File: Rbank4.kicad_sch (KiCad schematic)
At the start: 100 parts, among them K10 TQ2-5, K11 TQ2-5, K12 TQ2-5, K13 TQ2-5, K14 TQ2-5, K15 TQ2-5, K16 TQ2-5, K17 TQ2-5, K18 TQ2-5, Q10 2N2222, Q11 2N2222, Q12 2N2222, Q13 2N2222, Q14 2N2222, Q15 2N2222, Q16 2N2222, Q17 2N2222, Q18 2N2222

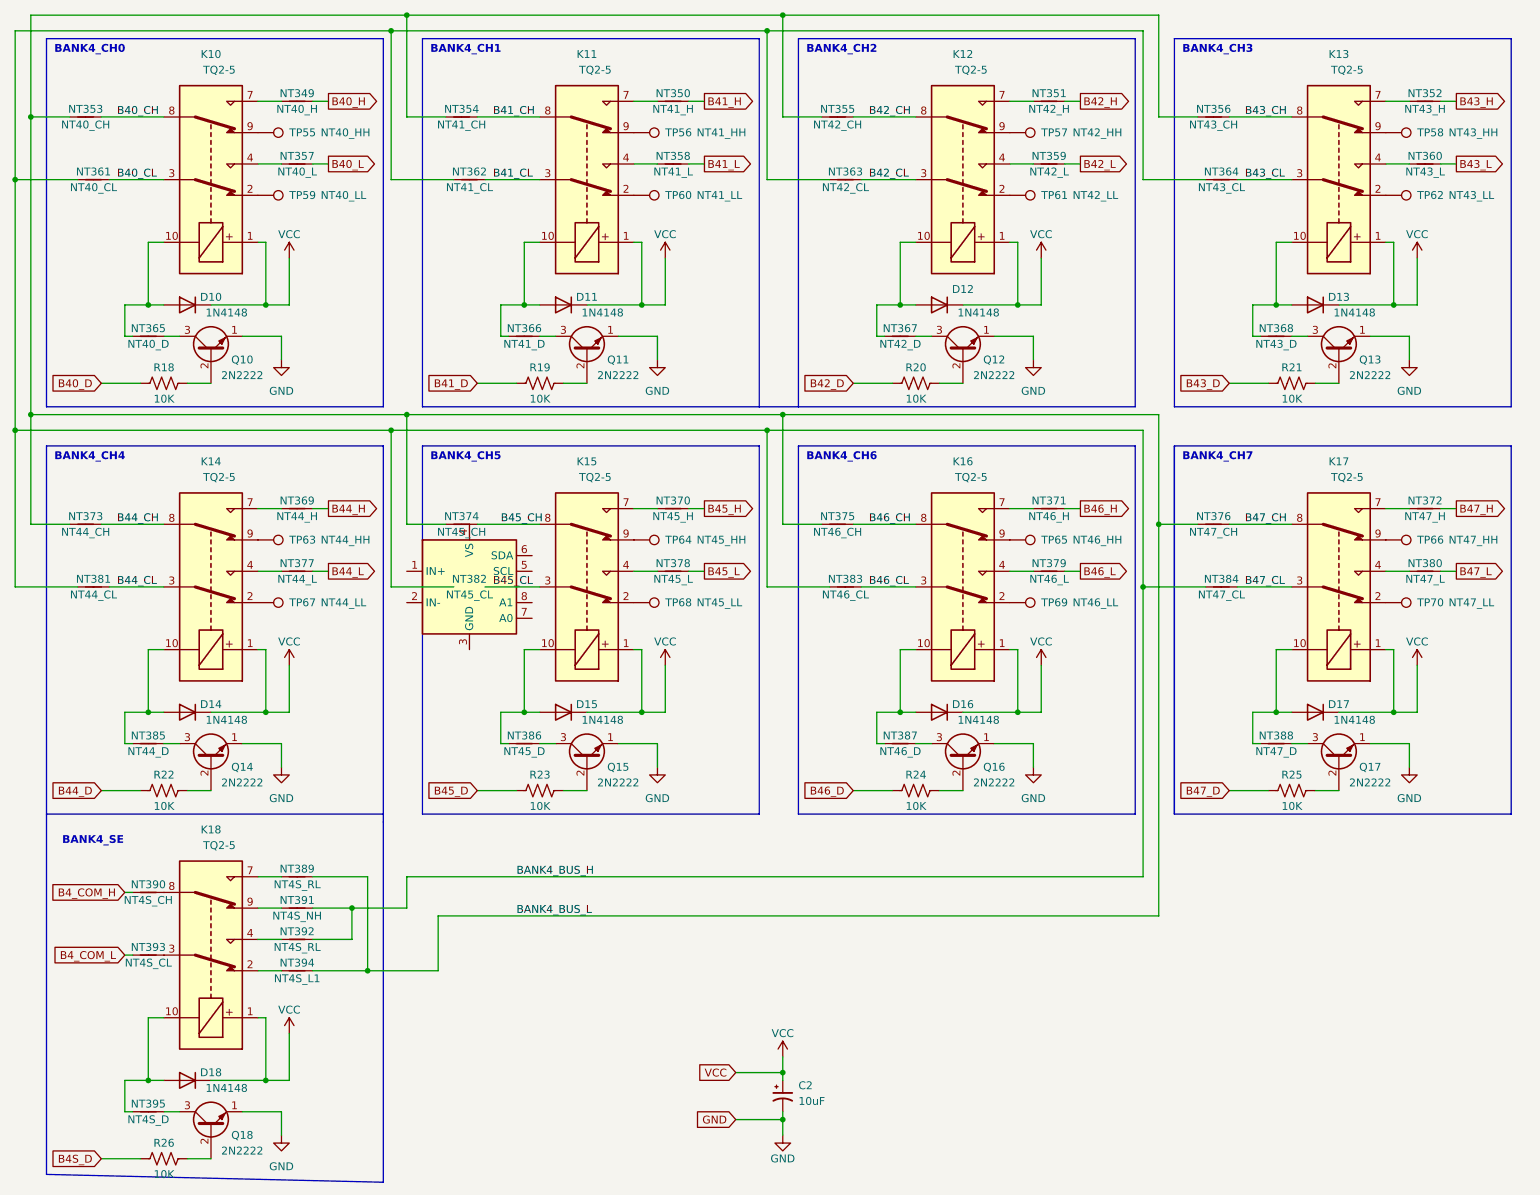
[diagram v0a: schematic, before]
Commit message: backup 1 bank done
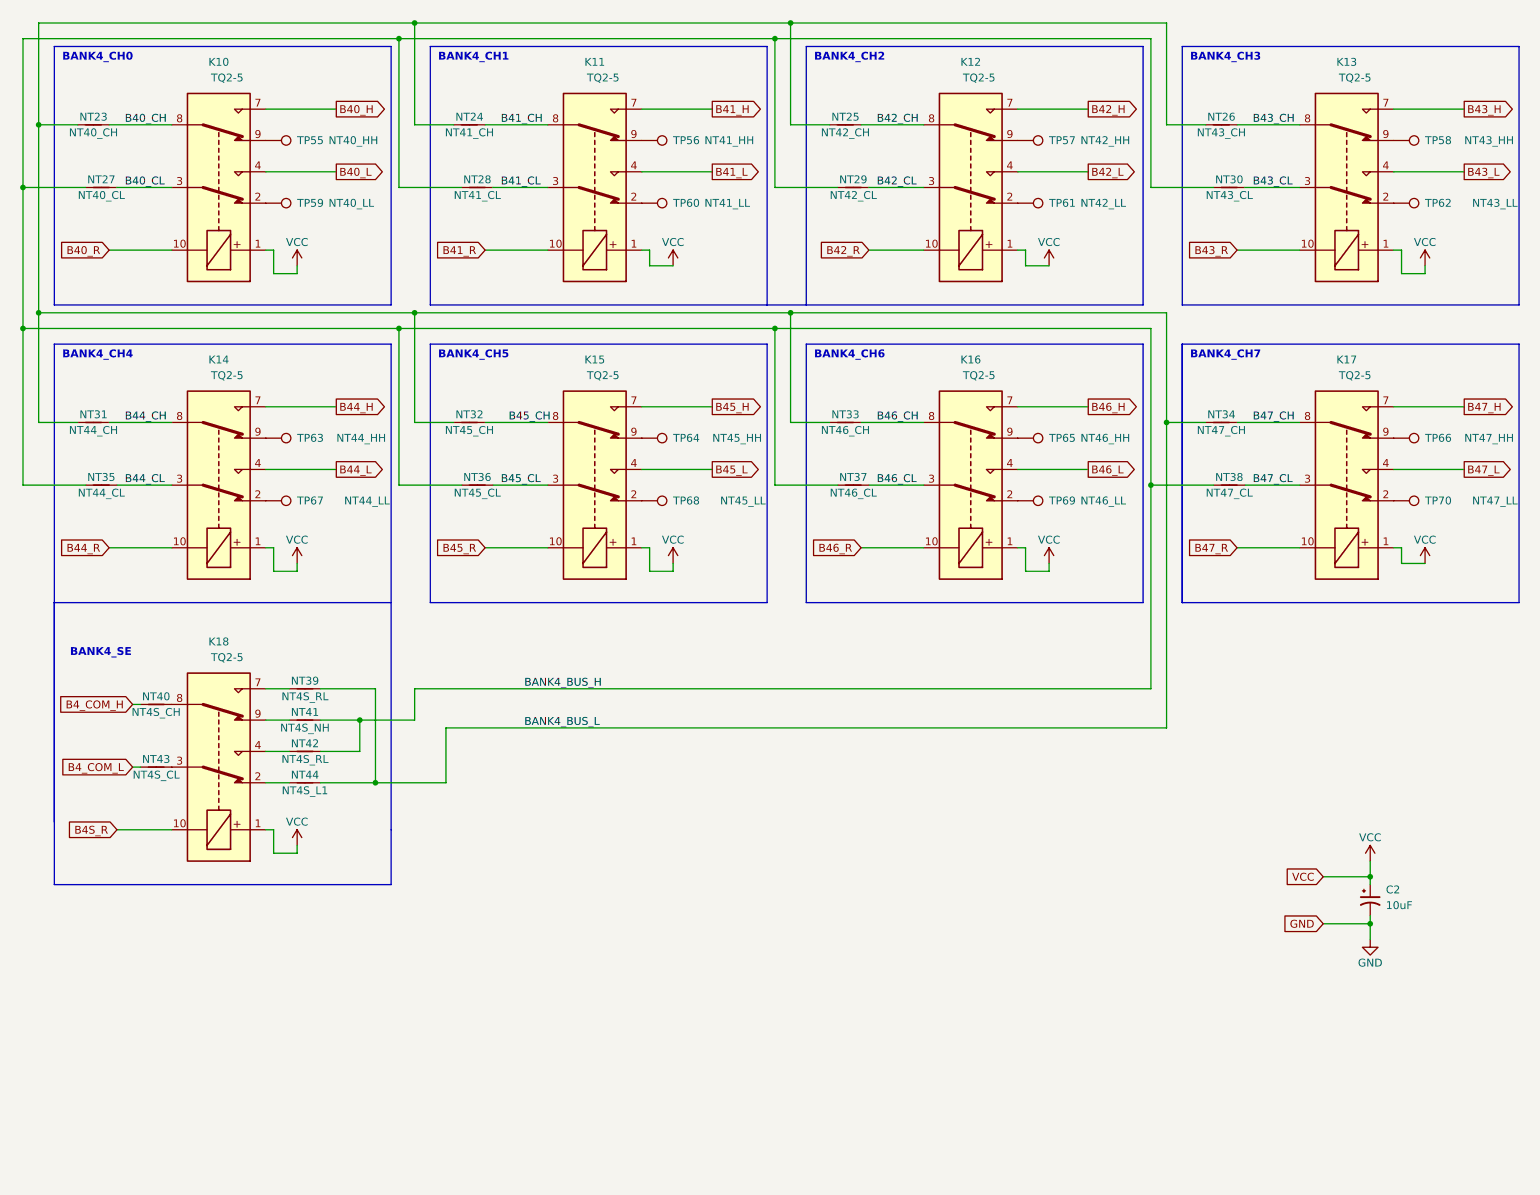
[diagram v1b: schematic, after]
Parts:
- removed D10, D11, D12, D13, D14, D15, D16, D17, D18: 1N4148, Diode_THT:D_DO-35_SOD27_P7.62mm_Horizontal, symbol Diode:1N4148
- removed NT349: NT40_H, NetTie:NetTie-2_THT_Pad1.0mm, symbol Device:NetTie_2
- removed NT350: NT41_H, NetTie:NetTie-2_THT_Pad1.0mm, symbol Device:NetTie_2
- removed NT351: NT42_H, NetTie:NetTie-2_THT_Pad1.0mm, symbol Device:NetTie_2
- removed NT352: NT43_H, NetTie:NetTie-2_THT_Pad1.0mm, symbol Device:NetTie_2
- removed NT353: NT40_CH, NetTie:NetTie-2_THT_Pad1.0mm, symbol Device:NetTie_2
- removed NT354: NT41_CH, NetTie:NetTie-2_THT_Pad1.0mm, symbol Device:NetTie_2
- removed NT355: NT42_CH, NetTie:NetTie-2_THT_Pad1.0mm, symbol Device:NetTie_2
- removed NT356: NT43_CH, NetTie:NetTie-2_THT_Pad1.0mm, symbol Device:NetTie_2
- removed NT357: NT40_L, NetTie:NetTie-2_THT_Pad1.0mm, symbol Device:NetTie_2
- removed NT358: NT41_L, NetTie:NetTie-2_THT_Pad1.0mm, symbol Device:NetTie_2
- removed NT359: NT42_L, NetTie:NetTie-2_THT_Pad1.0mm, symbol Device:NetTie_2
- removed NT360: NT43_L, NetTie:NetTie-2_THT_Pad1.0mm, symbol Device:NetTie_2
- removed NT361: NT40_CL, NetTie:NetTie-2_THT_Pad1.0mm, symbol Device:NetTie_2
- removed NT362: NT41_CL, NetTie:NetTie-2_THT_Pad1.0mm, symbol Device:NetTie_2
- removed NT363: NT42_CL, NetTie:NetTie-2_THT_Pad1.0mm, symbol Device:NetTie_2
- removed NT364: NT43_CL, NetTie:NetTie-2_THT_Pad1.0mm, symbol Device:NetTie_2
- removed NT365: NT40_D, NetTie:NetTie-2_THT_Pad1.0mm, symbol Device:NetTie_2
- removed NT366: NT41_D, NetTie:NetTie-2_THT_Pad1.0mm, symbol Device:NetTie_2
- removed NT367: NT42_D, NetTie:NetTie-2_THT_Pad1.0mm, symbol Device:NetTie_2
- removed NT368: NT43_D, NetTie:NetTie-2_THT_Pad1.0mm, symbol Device:NetTie_2
- removed NT369: NT44_H, NetTie:NetTie-2_THT_Pad1.0mm, symbol Device:NetTie_2
- removed NT370: NT45_H, NetTie:NetTie-2_THT_Pad1.0mm, symbol Device:NetTie_2
- removed NT371: NT46_H, NetTie:NetTie-2_THT_Pad1.0mm, symbol Device:NetTie_2
- removed NT372: NT47_H, NetTie:NetTie-2_THT_Pad1.0mm, symbol Device:NetTie_2
- removed NT373: NT44_CH, NetTie:NetTie-2_THT_Pad1.0mm, symbol Device:NetTie_2
- removed NT374: NT45_CH, NetTie:NetTie-2_THT_Pad1.0mm, symbol Device:NetTie_2
- removed NT375: NT46_CH, NetTie:NetTie-2_THT_Pad1.0mm, symbol Device:NetTie_2
- removed NT376: NT47_CH, NetTie:NetTie-2_THT_Pad1.0mm, symbol Device:NetTie_2
- removed NT377: NT44_L, NetTie:NetTie-2_THT_Pad1.0mm, symbol Device:NetTie_2
- removed NT378: NT45_L, NetTie:NetTie-2_THT_Pad1.0mm, symbol Device:NetTie_2
- removed NT379: NT46_L, NetTie:NetTie-2_THT_Pad1.0mm, symbol Device:NetTie_2
- removed NT380: NT47_L, NetTie:NetTie-2_THT_Pad1.0mm, symbol Device:NetTie_2
- removed NT381: NT44_CL, NetTie:NetTie-2_THT_Pad1.0mm, symbol Device:NetTie_2
- removed NT382: NT45_CL, NetTie:NetTie-2_THT_Pad1.0mm, symbol Analog_ADC:INA219AxDCN
- removed NT383: NT46_CL, NetTie:NetTie-2_THT_Pad1.0mm, symbol Device:NetTie_2
- removed NT384: NT47_CL, NetTie:NetTie-2_THT_Pad1.0mm, symbol Device:NetTie_2
- removed NT385: NT44_D, NetTie:NetTie-2_THT_Pad1.0mm, symbol Device:NetTie_2
- removed NT386: NT45_D, NetTie:NetTie-2_THT_Pad1.0mm, symbol Device:NetTie_2
- removed NT387: NT46_D, NetTie:NetTie-2_THT_Pad1.0mm, symbol Device:NetTie_2
- removed NT388: NT47_D, NetTie:NetTie-2_THT_Pad1.0mm, symbol Device:NetTie_2
- removed NT389, NT392: NT4S_RL, NetTie:NetTie-2_THT_Pad1.0mm, symbol Device:NetTie_2
- removed NT390: NT4S_CH, NetTie:NetTie-2_THT_Pad1.0mm, symbol Device:NetTie_2
- removed NT391: NT4S_NH, NetTie:NetTie-2_THT_Pad1.0mm, symbol Device:NetTie_2
- removed NT393: NT4S_CL, NetTie:NetTie-2_THT_Pad1.0mm, symbol Device:NetTie_2
- removed NT394: NT4S_L1, NetTie:NetTie-2_THT_Pad1.0mm, symbol Device:NetTie_2
- removed NT395: NT4S_D, NetTie:NetTie-2_THT_Pad1.0mm, symbol Device:NetTie_2
- removed Q10, Q11, Q12, Q13, Q14, Q15, Q16, Q17, Q18: 2N2222, Package_TO_SOT_THT:TO-92_Inline, symbol Transistor_BJT:2N3904
- removed R18, R19, R20, R21, R22, R23, R24, R25, R26: 10K, Resistor_THT:R_Axial_DIN0309_L9.0mm_D3.2mm_P12.70mm_Horizontal, symbol Device:R_US
- added NT23: NT40_CH, NetTie:NetTie-2_Front1.0mm, symbol Device:NetTie_2
- added NT24: NT41_CH, NetTie:NetTie-2_Front1.0mm, symbol Device:NetTie_2
- added NT25: NT42_CH, NetTie:NetTie-2_Front1.0mm, symbol Device:NetTie_2
- added NT26: NT43_CH, NetTie:NetTie-2_Front1.0mm, symbol Device:NetTie_2
- added NT27: NT40_CL, NetTie:NetTie-2_Front1.0mm, symbol Device:NetTie_2
- added NT28: NT41_CL, NetTie:NetTie-2_Front1.0mm, symbol Device:NetTie_2
- added NT29: NT42_CL, NetTie:NetTie-2_Front1.0mm, symbol Device:NetTie_2
- added NT30: NT43_CL, NetTie:NetTie-2_Front1.0mm, symbol Device:NetTie_2
- added NT31: NT44_CH, NetTie:NetTie-2_Front1.0mm, symbol Device:NetTie_2
- added NT32: NT45_CH, NetTie:NetTie-2_Front1.0mm, symbol Device:NetTie_2
- added NT33: NT46_CH, NetTie:NetTie-2_Front1.0mm, symbol Device:NetTie_2
- added NT34: NT47_CH, NetTie:NetTie-2_Front1.0mm, symbol Device:NetTie_2
- added NT35: NT44_CL, NetTie:NetTie-2_Front1.0mm, symbol Device:NetTie_2
- added NT36: NT45_CL, NetTie:NetTie-2_Front1.0mm, symbol Device:NetTie_2
- added NT37: NT46_CL, NetTie:NetTie-2_Front1.0mm, symbol Device:NetTie_2
- added NT38: NT47_CL, NetTie:NetTie-2_Front1.0mm, symbol Device:NetTie_2
- added NT39, NT42: NT4S_RL, NetTie:NetTie-2_Front1.0mm, symbol Device:NetTie_2
- added NT40: NT4S_CH, NetTie:NetTie-2_Front1.0mm, symbol Device:NetTie_2
- added NT41: NT4S_NH, NetTie:NetTie-2_Front1.0mm, symbol Device:NetTie_2
- added NT43: NT4S_CL, NetTie:NetTie-2_Front1.0mm, symbol Device:NetTie_2
- added NT44: NT4S_L1, NetTie:NetTie-2_Front1.0mm, symbol Device:NetTie_2
- TP55, TP56, TP57, TP58, TP59, TP60, TP61, TP62, TP63, TP64, TP65, TP66, TP67, TP68, TP69, TP70: footprint Connector_Pin:Pin_D1.0mm_L10.0mm -> Connector_Pin:Pin_D0.9mm_L10.0mm_W2.4mm_FlatFork
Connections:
- net B40_CH: now also NT23.2
- net B40_CL: now also NT27.2
- net B40_H: now also K10.7
- net B40_L: now also K10.4
- net B41_CH: now also NT24.2
- net B41_CL: now also NT28.2
- net B41_H: now also K11.7
- net B41_L: now also K11.4
- net B42_CH: now also NT25.2
- net B42_CL: now also NT29.2
- net B42_H: now also K12.7
- net B42_L: now also K12.4
- net B43_CH: now also NT26.2
- net B43_CL: now also NT30.2
- net B43_H: now also K13.7
- net B43_L: now also K13.4
- net B44_CH: now also NT31.2
- net B44_CL: now also NT35.2
- net B44_H: now also K14.7
- net B44_L: now also K14.4
- net B45_CH: now also NT32.2
- net B45_CL: now also NT36.2
- net B45_H: now also K15.7
- net B45_L: now also K15.4
- net B46_CH: now also NT33.2
- net B46_CL: now also NT37.2
- net B46_H: now also K16.7
- net B46_L: now also K16.4
- net B47_CH: now also NT34.2
- net B47_CL: now also NT38.2
- net B47_H: now also K17.7
- net B47_L: now also K17.4
- net B4_COM_H: now also NT40.1
- net B4_COM_L: now also NT43.1
- net BANK4_BUS_H: now also NT27.1, NT28.1, NT29.1, NT30.1, NT35.1, NT36.1, NT37.1, NT38.1, NT41.2, NT42.2
- net BANK4_BUS_L: now also NT23.1, NT24.1, NT25.1, NT26.1, NT31.1, NT32.1, NT33.1, NT34.1, NT39.2, NT44.2
- net B42_R: now reaches K12.10
- net B43_R: now reaches K13.10
- net B41_R: now reaches K11.10
- net B47_R: now reaches K17.10
- net B4S_R: now reaches K18.10
- net at K18.2: now also NT44.1
- net at K18.3: now also NT43.2
- net at K18.4: now also NT42.1
- net at K18.7: now also NT39.1
- net at K18.8: now also NT40.2
- net at K18.9: now also NT41.1
- net B45_R: now reaches K15.10
- net B40_R: now reaches K10.10
- net B46_R: now reaches K16.10
- net B44_R: now reaches K14.10

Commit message: PCB Completed
PCB completed but final verification not completed
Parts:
- TP55, TP56, TP57, TP58, TP59, TP60, TP61, TP62, TP63, TP64, TP65, TP66, TP67, TP68, TP69, TP70: footprint Connector_Pin:Pin_D0.9mm_L10.0mm_W2.4mm_FlatFork -> TestPoint:TestPoint_THTPad_D1.5mm_Drill0.7mm
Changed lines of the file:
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@@
       (effects (font (size 1.27 1.27)) (justify left))
     )
-    (property "Footprint" "Connector_Pin:Pin_D0.9mm_L10.0mm_W2.4mm_FlatFork" (id 2) (at 238.76 87.63 0)
+    (property "Footprint" "TestPoint:TestPoint_THTPad_D1.5mm_Drill0.7mm" (id 2) (at 238.76 87.63 0)
       (effects (font (size 1.27 1.27)) hide)
     )
@@
       (effects (font (size 1.27 1.27)) (justify left))
     )
-    (property "Footprint" "Connector_Pin:Pin_D0.9mm_L10.0mm_W2.4mm_FlatFork" (id 2) (at 55.88 39.37 0)
+    (property "Footprint" "TestPoint:TestPoint_THTPad_D1.5mm_Drill0.7mm" (id 2) (at 55.88 39.37 0)
       (effects (font (size 1.27 1.27)) hide)
     )
@@
       (effects (font (size 1.27 1.27)) (justify left))
     )
-    (property "Footprint" "Connector_Pin:Pin_D0.9mm_L10.0mm_W2.4mm_FlatFork" (id 2) (at 238.76 49.53 0)
+    (property "Footprint" "TestPoint:TestPoint_THTPad_D1.5mm_Drill0.7mm" (id 2) (at 238.76 49.53 0)
       (effects (font (size 1.27 1.27)) hide)
     )
@@
       (effects (font (size 1.27 1.27)) (justify left))
     )
-    (property "Footprint" "Connector_Pin:Pin_D0.9mm_L10.0mm_W2.4mm_FlatFork" (id 2) (at 238.76 97.79 0)
+    (property "Footprint" "TestPoint:TestPoint_THTPad_D1.5mm_Drill0.7mm" (id 2) (at 238.76 97.79 0)
       (effects (font (size 1.27 1.27)) hide)
     )
@@
       (effects (font (size 1.27 1.27)) (justify left))
     )
-    (property "Footprint" "Connector_Pin:Pin_D0.9mm_L10.0mm_W2.4mm_FlatFork" (id 2) (at 116.84 97.79 0)
+    (property "Footprint" "TestPoint:TestPoint_THTPad_D1.5mm_Drill0.7mm" (id 2) (at 116.84 97.79 0)
       (effects (font (size 1.27 1.27)) hide)
     )
@@
       (effects (font (size 1.27 1.27)) (justify left))
     )
-    (property "Footprint" "Connector_Pin:Pin_D0.9mm_L10.0mm_W2.4mm_FlatFork" (id 2) (at 55.88 49.53 0)
+    (property "Footprint" "TestPoint:TestPoint_THTPad_D1.5mm_Drill0.7mm" (id 2) (at 55.88 49.53 0)
       (effects (font (size 1.27 1.27)) hide)
     )
@@
       (effects (font (size 1.27 1.27)) (justify left))
     )
-    (property "Footprint" "Connector_Pin:Pin_D0.9mm_L10.0mm_W2.4mm_FlatFork" (id 2) (at 55.88 87.63 0)
+    (property "Footprint" "TestPoint:TestPoint_THTPad_D1.5mm_Drill0.7mm" (id 2) (at 55.88 87.63 0)
       (effects (font (size 1.27 1.27)) hide)
     )
@@
       (effects (font (size 1.27 1.27)) (justify left))
     )
-    (property "Footprint" "Connector_Pin:Pin_D0.9mm_L10.0mm_W2.4mm_FlatFork" (id 2) (at 177.8 39.37 0)
+    (property "Footprint" "TestPoint:TestPoint_THTPad_D1.5mm_Drill0.7mm" (id 2) (at 177.8 39.37 0)
       (effects (font (size 1.27 1.27)) hide)
     )
@@
       (effects (font (size 1.27 1.27)) (justify left))
     )
-    (property "Footprint" "Connector_Pin:Pin_D0.9mm_L10.0mm_W2.4mm_FlatFork" (id 2) (at 177.8 97.79 0)
+    (property "Footprint" "TestPoint:TestPoint_THTPad_D1.5mm_Drill0.7mm" (id 2) (at 177.8 97.79 0)
       (effects (font (size 1.27 1.27)) hide)
     )
@@
       (effects (font (size 1.27 1.27)) (justify left))
     )
-    (property "Footprint" "Connector_Pin:Pin_D0.9mm_L10.0mm_W2.4mm_FlatFork" (id 2) (at 177.8 87.63 0)
+    (property "Footprint" "TestPoint:TestPoint_THTPad_D1.5mm_Drill0.7mm" (id 2) (at 177.8 87.63 0)
       (effects (font (size 1.27 1.27)) hide)
     )
@@
       (effects (font (size 1.27 1.27)) (justify left))
     )
-    (property "Footprint" "Connector_Pin:Pin_D0.9mm_L10.0mm_W2.4mm_FlatFork" (id 2) (at 116.84 49.53 0)
+    (property "Footprint" "TestPoint:TestPoint_THTPad_D1.5mm_Drill0.7mm" (id 2) (at 116.84 49.53 0)
       (effects (font (size 1.27 1.27)) hide)
     )
@@
       (effects (font (size 1.27 1.27)) (justify left))
     )
-    (property "Footprint" "Connector_Pin:Pin_D0.9mm_L10.0mm_W2.4mm_FlatFork" (id 2) (at 116.84 39.37 0)
+    (property "Footprint" "TestPoint:TestPoint_THTPad_D1.5mm_Drill0.7mm" (id 2) (at 116.84 39.37 0)
       (effects (font (size 1.27 1.27)) hide)
     )
@@
       (effects (font (size 1.27 1.27)) (justify left))
     )
-    (property "Footprint" "Connector_Pin:Pin_D0.9mm_L10.0mm_W2.4mm_FlatFork" (id 2) (at 55.88 97.79 0)
+    (property "Footprint" "TestPoint:TestPoint_THTPad_D1.5mm_Drill0.7mm" (id 2) (at 55.88 97.79 0)
       (effects (font (size 1.27 1.27)) hide)
     )
@@
       (effects (font (size 1.27 1.27)) (justify left))
     )
-    (property "Footprint" "Connector_Pin:Pin_D0.9mm_L10.0mm_W2.4mm_FlatFork" (id 2) (at 177.8 49.53 0)
+    (property "Footprint" "TestPoint:TestPoint_THTPad_D1.5mm_Drill0.7mm" (id 2) (at 177.8 49.53 0)
       (effects (font (size 1.27 1.27)) hide)
     )
@@
       (effects (font (size 1.27 1.27)) (justify left))
     )
-    (property "Footprint" "Connector_Pin:Pin_D0.9mm_L10.0mm_W2.4mm_FlatFork" (id 2) (at 116.84 87.63 0)
+    (property "Footprint" "TestPoint:TestPoint_THTPad_D1.5mm_Drill0.7mm" (id 2) (at 116.84 87.63 0)
       (effects (font (size 1.27 1.27)) hide)
     )
@@
       (effects (font (size 1.27 1.27)) (justify left))
     )
-    (property "Footprint" "Connector_Pin:Pin_D0.9mm_L10.0mm_W2.4mm_FlatFork" (id 2) (at 238.76 39.37 0)
-      (effects (font (size 1.27 1.27)) hide)
-    )
+    (property "Footprint" "TestPoint:TestPoint_THTPad_D1.5mm_Drill0.7mm" (id 2) (at 238.76 39.37 0)
+      (effects (font (size 1.27 1.27)) hide)
+    )
